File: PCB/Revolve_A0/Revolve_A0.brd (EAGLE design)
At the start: 100 x 100 mm, 366 parts, among them IC29 LAN8710A, IC30 MTFC2GMDEA, IC6 74AHC1G126DCK, IC7 74AHC1G126DCK, Q1 AON6758, Q2 AON6758, Q3 AON6758, Q8 AON6758, Q9 MMBT2907, U1 OSD3358-512M-BSM, U10 TPD4S012_DRY_6, U19 CD4050BD, U2 TUSB2046BIRHBT, U3 TPD2E001DRSR, U4 TPD2E001DRSR, U7 TLVH431, X1 22-05-7038-03, X10 22-05-7038-03, X11 22-05-7038-03, X12 22-05-7048-04, X13 22-05-7038-03, X14 22-05-7048-04, X15 22-05-7048-04, X16 22-05-7048-04, X17 22-05-7048-04, X18 22-05-7048-04, X19 22-05-7038-03, X2 MSTBA4, X20 MSTBA4, X21 MSTBA2, X22 22-05-7038-03, X24 HDMI, X25 22-05-7048-04, X26 MSTBA2, X29 22-05-7038-03, X3 MSTBA2, X4 22-05-7028-02, X5 22-05-7028-02, X6 22-05-7028-02, X7 22-05-7038-03, X8 22-05-7038-03, X9 22-05-7028-02, Y1 25MHz, Y2 25MHz, Y4 6 MHz

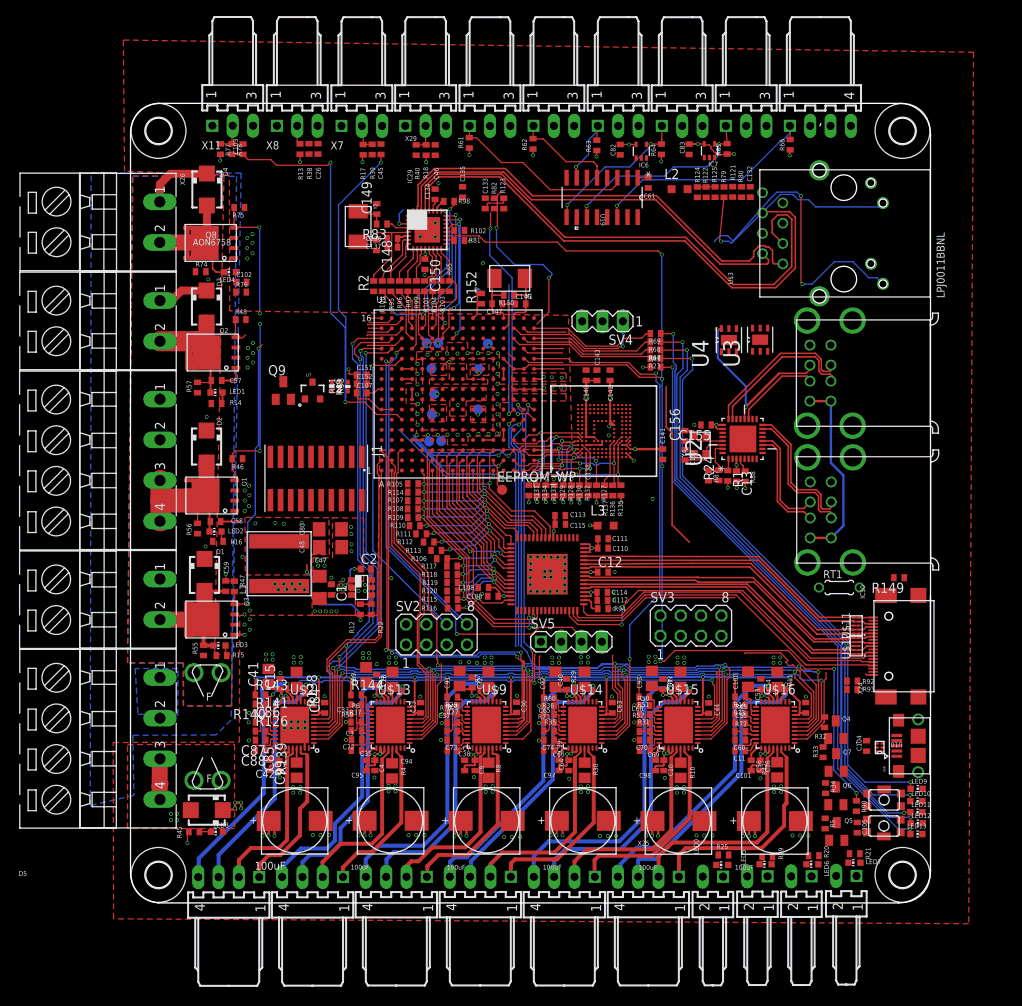
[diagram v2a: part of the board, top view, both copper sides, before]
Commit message: Almost done with schematic
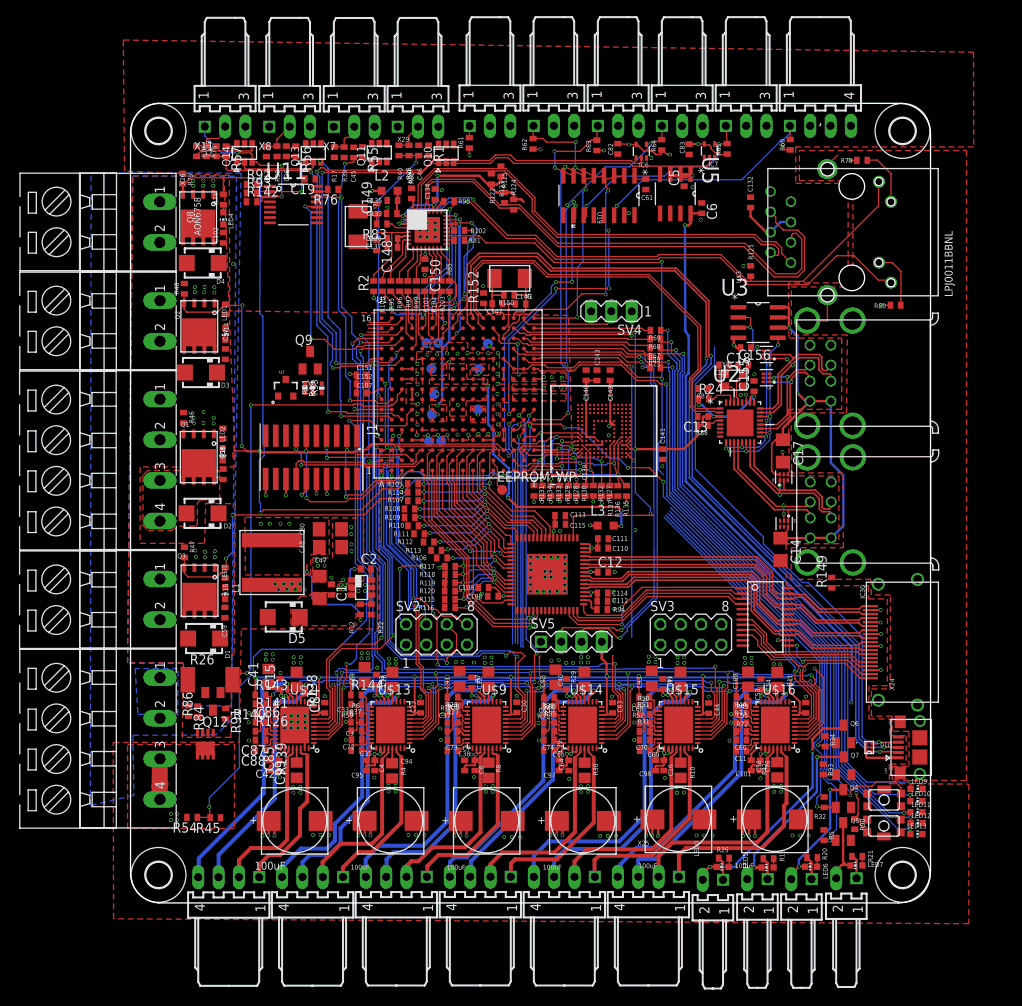
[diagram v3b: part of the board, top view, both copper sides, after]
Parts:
- removed C104, C105: 0.1uF, rcl:C0402
- removed F1: FUSE, fuse:3557
- removed FH1, FH2: FUSE-HOLDER, Replicape_Rev_B0:FUSE-HOLDER
- removed LED8: blue, led:CHIP-LED0603
- removed RT1: (no value), rcl:0204/5
- removed U$11, U$12: DF10G7M1N, Revolve:DF10G7M1N
- added C14, C17: 22uF, rcl:C1206
- added C18, C19, C5, C6: 0.1uF, rcl:C0402
- added Q10, Q11, Q13, Q14: DMC2038LVT, Manga_screen_rev_B:TSOT26
- added Q12: (no value), semicon-smd-ipc:SOT23
- added R142, R54, R91: 4.7K, rcl:R0402
- added R26: 0.001,1%, resistor:R2512
- added R84, R86: 100K,1%, rcl:R0402
- added U$17: SISS27DN, Revolve:POWERPAK-1212-8S
- added U$18: TPD12S016-RKT, Revolve:R-PDSO-G24
- added U11: SN74AHC595PW, Replicape_B3:SOP65P640X120-16N
- added U5: UA78L05ACD, Texas Instruments_By_element14_Batch_1:SOIC127P600X175-8N
- added U6, U8, U9: TPD4S012_DRY_6_P1_P, OSD3358-SM-RED Platform:DRY6
- C148, C149: value 30pF -> 18pF
- R1: value 1.5K -> 10K
- R105, R106, R107, R108, R109, R110, R111, R112, R113, R114, R115, R116, R117, R118, R119, R120: value 100K -> 100K,1%
- R2: value 0,DNI -> 0R,DNI
- R45: value 4.7K -> 100K,1%
- R55, R56, R57: value 4.7K -> 10K
- U3: value TPD2E001DRSR -> TPS2061D; device Texas Instruments_By_element14_Batch_1:SON95P315X315X80-7N -> Texas Instruments_By_element14_Batch_1:SOIC127P600X175-8N
- U4: value TPD2E001DRSR -> TPD4S012_DRY_6_P1_P; device Texas Instruments_By_element14_Batch_1:SON95P315X315X80-7N -> OSD3358-SM-RED Platform:DRY6
- X24: value HDMI -> HDMI4; device hdmi:HDMI-C -> hdmi:HDMI-A-TH
- moved R93 97.4 mm to (15.2, 88.8)
- moved R92 97.4 mm to (15.2, 89.8)
- moved R55 65.4 mm to (29.0, 93.8)
- moved R1 55.2 mm to (37.2, 94.0)
- moved R56 48.7 mm to (20.6, 94.0)
- moved L2 36.3 mm to (32.4, 89.0)
- moved R57 29.7 mm to (11.9, 94.0)
- moved R122 26.9 mm to (45.1, 90.5), turned to 90 degrees
- moved R125 26.3 mm to (46.8, 88.2)
- moved D5 26.0 mm to (19.1, 35.8)
- moved R80 23.9 mm to (95.6, 74.7), turned to 180 degrees
- moved R124 23.0 mm to (47.9, 87.3)
- moved R79 17.7 mm to (91.4, 92.8), turned to 180 degrees
- moved R76 17.2 mm to (25.3, 89.2), turned to 180 degrees
- moved R16 13.5 mm to (11.6, 58.7), turned to 90 degrees
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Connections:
- net N$152 renamed VDDCR
- net N$25 renamed RTC_KALDO_ENN
- net TK_HBP renamed I_MEASURE
- removed net DDC/CEC-GRND: X24.17
- removed net ECAP1: SV5.3, U1.B12
- removed net ECAP2: SV5.2, U1.A12
- removed net EHRPWM1A: U1.P12
- removed net EHRPWM1B: U1.T13
- removed net EHRPWM2A: U1.T4
- removed net EHRPWM2B: U1.P5
- removed net GPIO0_18: U1.J15
- removed net GPIO0_26: U1.R5
- removed net N$17: U2.10, U2.14, U2.18, U2.22
- removed net N$193: U$5.3, U2.12
- removed net N$194: U$5.2, U2.11
- removed net N$195: U$5.7, U2.16
- removed net N$196: U$5.6, U2.15
- removed net SPI0_CSE: U$14.2, U1.T12
- removed net SPI0_CSH: U$15.2, U1.R7
- removed net SPI0_CSX: U$2.2, U1.A14
- removed net SPI0_CSY: U$13.2, U1.C14
- removed net SPI0_CSZ: U$9.2, U1.T7
- removed net TIMER4: U1.M1
- removed net TIMER5: U1.N3
- removed net TIMER6: U1.N2
- removed net TIMER7: U1.N1
- removed net TK_A: U1.D7
- removed net USB_HOST_5V: U$5.1, U$5.5, U$6.1, U$6.5
- removed net VCC: U3.1, U4.1
- new net +12V: C5.2, U5.1, X12.4
- new net +24V_FOR_5V: C1.2, C47.1, D5.C, U$10.3
- new net ENABLE_STUFF: Q12.1, R91.1, U1.J15
- new net EN_TK_A: Q14.1, Q14.3, R142.2, U11.3, X11.1
- new net EN_TK_E: Q10.1, Q10.3, R76.2, U11.15, X29.1
- new net EN_TK_H: Q11.1, Q11.3, R92.2, U11.1, X7.1
- new net EN_TK_HBP: Q13.1, Q13.3, R93.2, U11.2, X8.1
- new net MGND: C102.2, C57.2, C58.2, C59.2, LED1.C, LED2.C, LED3.C, LED4.C, Q1.1, Q1.2, Q1.3, Q2.1, Q2.2, Q2.3, Q3.1, Q3.2, Q3.3, Q8.1, Q8.2, Q8.3, R26.2, R46.1, R47.1, R48.1, R75.1
- new net N$26: R84.2, R86.1, U$17.G
- new net N$31: U$18.P$10, X24.19
- new net N$33: Q10.6, R1.1
- new net N$47: Q10.4, R18.2
- new net N$50: Q13.6, R56.1
- new net N$53: Q14.6, R57.1
- new net N$55: U$18.P$9, X24.16
- new net N$56: U$18.P$8, X24.15
- new net N$57: U$18.P$7, X24.13
- new net N$58: Q11.4, R17.2
- new net N$59: Q13.4, R13.2
- new net N$60: Q14.4, R77.2
- new net N$65: Q11.6, R55.1
- new net SPI0_CS0: U$13.2, U$14.2, U$15.2, U$16.2, U$2.2, U$9.2, U1.A14
- new net SPI0_CS1: U1.C14, U11.12
- new net SPI0_MISO_E: U$14.5, U$15.4
- new net SPI0_MISO_H: U$15.5, U$16.4
- new net SPI0_MISO_X: U$13.4, U$2.5
- new net SPI0_MISO_Y: U$13.5, U$9.4
- new net SPI0_MISO_Z: U$14.4, U$9.5
- new net USB1_DM1: U$5.2, U2.11, U9.1
- new net USB1_DM2: U$5.6, U2.15, U6.1
- new net USB1_DP1: U$5.3, U2.12, U9.2
- new net USB1_DP2: U$5.7, U2.16, U6.2
- new net USB1_DRVVBUS: U1.M14
- new net USB_OC: U2.10, U2.14, U2.18, U2.22, U3.5
- new net USB_PWR: U2.9, U3.2, U3.3
- new net USB_VBUS: C14.1, C17.1, U$5.1, U$5.5, U$6.1, U$6.5, U3.6, U3.7, U3.8, U4.6, U6.6, U8.6, U9.6
- new net VIN_MEASURE: R45.2, R54.1, U1.D7
- net +24V: now also C6.2, U$17.S1, U$17.S2, U$17.S3, U5.8; no longer C1.2, C47.1, D5.C, F1.P$3, F1.P$4, R14.2, R15.2, R16.2, R45.1, R55.2, R56.2, R57.2, R74.2, R76.2, U$10.3, X12.4
- net +5V: now also C18.2, C19.1, U$18.P$11, U1.M15, U11.10, U11.16, U3.4
- net CGND: now also X24.P$1, X24.P$2, X24.P$3, X24.P$4; no longer X24.PAD1, X24.PAD2, X24.PAD3, X24.PAD4
- net DVI_+5V: now also U$18.P$13; no longer R92.2, R93.2, RT1.2
- net ENABLE_B: now also SV2.3, U1.T7; no longer SV2.4
- net ENABLE_C: now also U1.R7
- net FAN0: now also U1.P12
- net FAN1: now also U1.T13
- net FAN2: now also U1.T4
- net FAN3: now also U1.P5
- net FAULT_B: now also SV2.1, U1.T12; no longer SV2.2
- net FAULT_C: now also U1.R5
- net GND: now also C14.2, C17.2, C18.1, C19.2, C5.1, C6.1, Q10.5, Q11.5, Q12.2, Q13.5, Q14.5, R142.1, R26.1, R54.2, R76.1, R91.2, R92.1, R93.1, U$18.P$14, U$18.P$19, U$18.P$6, U1.L14, U11.13, U11.8, U3.1, U4.4, U5.2, U5.3, U5.6, U5.7, U6.4, U8.4, U9.4, X24.17; no longer C102.2, C104.2, C105.1, C57.2, C58.2, C59.2, D5.A, Q1.1, Q1.2, Q1.3, Q2.1, Q2.2, Q2.3, Q3.1, Q3.2, Q3.3, Q8.1, Q8.2, Q8.3, R46.1, R47.1, R48.1, R75.1, U$11.3, U$12.3
- net HDMI_HPD: now also U$18.P$4; no longer X24.19
- net HEATER_A: now also R74.2, U1.N1
- net HEATER_E: now also R15.2, U1.M1
- net HEATER_H: now also R14.2, U1.N3
- net HEATER_HBP: now also R16.2, U1.N2
- net N$150: no longer LED4.C, R76.1
- net N$169: now also U$18.P$1; no longer X24.13
- net N$207: now also U$18.P$2; no longer R92.1, X24.15
- net N$208: now also U$18.P$3; no longer R93.1, X24.16
- net N$234: no longer LED3.C, R55.1
- net N$242: no longer LED2.C, R56.1
- net N$64: no longer LED1.C, R57.1
- net N$8: now also Q12.3, R86.2; no longer LED8.C, R45.2
- net QUAD_ENCODER_A: now also SV5.3
- net QUAD_ENCODER_B: now also SV5.2
- net SERVO_0: now also U1.B12
- net SERVO_0_EN: now also U11.4
- net SERVO_1: now also U1.A12
- net SERVO_1_EN: now also U11.5
- net SPI0_CSA: no longer U$16.2
- net SPI0_MISO: no longer U$13.5, U$14.5, U$15.5, U$2.5, U$9.5
- net SPI0_MOSI: now also U11.14; no longer U$13.4, U$14.4, U$15.4, U$16.4, U$9.4
- net SPI0_SCLK: now also U11.11
- net SPI1_CS1: now also SV2.4; no longer SV2.3
- net SPI1_SCLK: now also SV2.2; no longer SV2.1
- net SYS_5V: no longer RT1.1, X11.1, X29.1, X7.1, X8.1
- net SYS_RESETN: no longer C105.2
- net SYS_VDD1_3V3: now also SV5.4, U$18.P$24; no longer R1.2
- net SYS_VDD2_3V3: no longer SV5.4
- net TERM_A: now also R57.2
- net TERM_E: now also R1.2
- net TERM_H: now also R56.2
- net TERM_HBP: now also R55.2
- net TX0+: now also U$18.P$18; no longer U$12.5, U$12.6
- net TX0-: now also U$18.P$17; no longer U$12.4, U$12.7
- net TX1+: now also U$18.P$21; no longer U$11.2, U$11.9
- net TX1-: now also U$18.P$20; no longer U$11.1, U$11.10
- net TX2+: now also U$18.P$23; no longer U$11.5, U$11.6
- net TX2-: now also U$18.P$22; no longer U$11.4, U$11.7
- net TXC+: now also U$18.P$16; no longer U$12.2, U$12.9
- net TXC-: now also U$18.P$15; no longer U$12.1, U$12.10
- net USB1_DM3: now also U4.1; no longer U4.3
- net USB1_DM4: now also U8.1; no longer U3.3
- net USB1_DP: no longer R1.1
- net USB1_DP3: now also U4.2; no longer U4.6
- net USB1_DP4: now also U8.2; no longer U3.6
- net USB_DC: no longer C104.1
- net VDD_ADC: now also Q10.2, Q11.2, Q13.2, Q14.2; no longer R13.2, R17.2, R18.2, R77.2
- net VIN: now also D5.A, R45.1, R84.1, U$17.D1, U$17.D2, U$17.D3, U$17.D4, U$17.D5; no longer F1.P$1, F1.P$2, LED8.A
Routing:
- net SPI0_CS0: track 0.00 -> 169.1 mm, vias 0 -> 8
- net SPI0_MISO: track 164.0 -> 36.8 mm, vias 7 -> 1
- net USB0_DP: track 0.00 -> 111.5 mm, vias 0 -> 2
- net SPI0_MOSI: track 170.6 -> 83.1 mm, vias 8 -> 3
- net STEP_H: track 13.3 -> 99.8 mm, vias 0 -> 2
- net N$179: track 3.72 -> 88.2 mm, vias 0 -> 2
- net USB0_DM: track 25.6 -> 109.1 mm, vias 1 -> 2
- net SERVO_1: track 0.00 -> 81.0 mm, vias 0 -> 2
- net FAN1: track 0.00 -> 79.5 mm, vias 0 -> 2
- net FAN3: track 0.00 -> 78.9 mm, vias 0 -> 4
- net SERVO_0: track 0.00 -> 76.4 mm, vias 0 -> 2
- net VIN_MEASURE: track 0.00 -> 75.5 mm, vias 0 -> 2
- net HEATER_A: track 16.7 -> 91.7 mm, vias 2 -> 4
- net N$156: track 0.00 -> 73.7 mm, vias 0 -> 2
- net SPI0_CSH: track 71.7 -> 0.00 mm, vias 2 -> 0
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- added copper zone on layer 3, net +12V
- added copper zone on layer 1, net +24V_FOR_5V
- added copper zone on layer 1, net CGND
- added copper zone on layer 1, net N$242
- added copper zone on layer 3, net N$42
- added copper zone on layer 3, net USB_DC
- removed copper zone on layer 3, net N$18
